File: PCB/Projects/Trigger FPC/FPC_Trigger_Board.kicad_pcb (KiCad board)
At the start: 2 copper layers, 127.6 x 29.7 mm, 10 parts, among them J1 Conn_01x05_Pin, J2 Conn_01x05_Pin, U1 HAL4395, U2 HAL4395, U3 HAL4395, U4 HAL4395

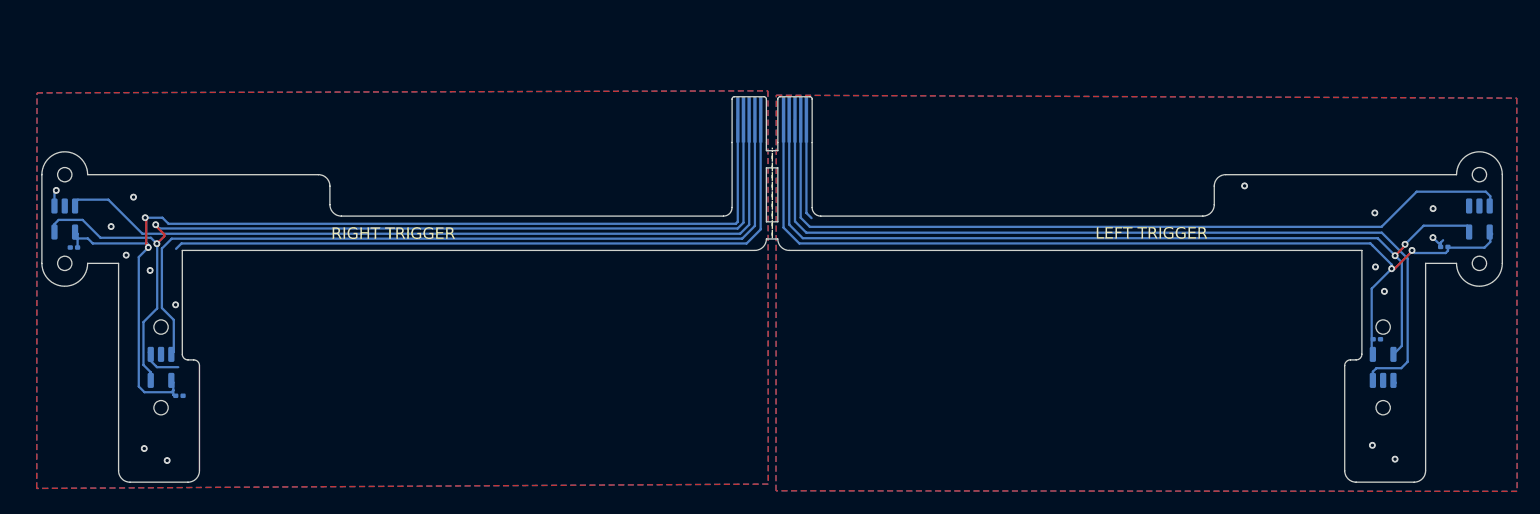
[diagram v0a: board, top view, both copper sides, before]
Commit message: FPC Board Update
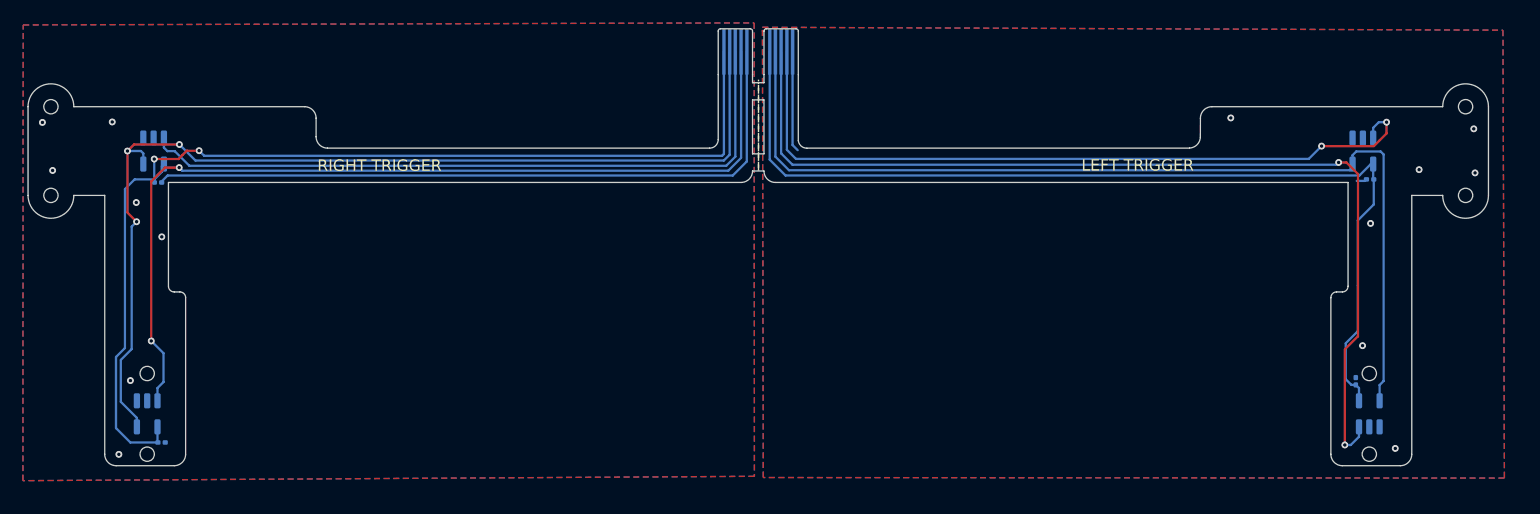
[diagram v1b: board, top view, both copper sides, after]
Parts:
- moved U2 11.8 mm to (270.3, 135.3)
- moved U4 9.78 mm to (164.6, 135.3)
- moved C4 9.29 mm to (165.0, 138.1), turned to 180 degrees
- moved C2 8.77 mm to (270.9, 137.8)
- moved J1 6.06 mm to (219.5, 126.6)
- moved J2 6.06 mm to (215.5, 126.6)
- moved C3 4.37 mm to (165.3, 160.8)
- moved U3 4.24 mm to (164.1, 158.3)
- moved U1 4.24 mm to (270.9, 158.3)
- moved C1 4.11 mm to (269.7, 155.4), turned to -90 degrees
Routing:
- net ADC_1: track 71.7 -> 81.7 mm, vias 0 -> 2
- net ADC_3: track 77.0 -> 86.8 mm, vias 0 -> 2
- net ADC_0: track 70.0 -> 60.9 mm
- net ADC_2: track 71.5 -> 65.5 mm, vias 0 -> 2
- net TRIGGER_EN_L: track 80.9 -> 85.9 mm, vias 2 -> 0
- net GND: track 66.3 -> 61.6 mm, vias 8 -> 7
- net TRIGGER_EN_R: track 86.3 -> 90.7 mm, vias 2 -> 3
- net +3V3: track 89.4 -> 92.7 mm
- net +3V3L: track 83.7 -> 85.6 mm, vias 2 -> 0
- net GNDL: track 10.9 -> 9.70 mm, vias 8 -> 7
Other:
- board size 127.6 x 29.7 mm -> 127.6 x 34.2 mm
